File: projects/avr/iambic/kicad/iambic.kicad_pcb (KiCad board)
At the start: 2 copper layers, 48.3 x 50.8 mm, 24 parts, among them P1 CONN_1, P2 CONN_1, P3 CONN_1, P4 CONN_1, P5 CONN_1, P6 CONN_1, P7 CONN_1, P8 CONN_6, P9 CONN_1, Q1 NPN, Q2 NPN, U1 ATTINY45-20PU

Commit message: add install-op-rockpi/kicad/mp3server
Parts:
- RV1, RV2: footprint kicad:PIN_ARRAY_3X1 -> kicad:POT_V
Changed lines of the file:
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@@
     (add_net "Net-(R6-Pad1)")
   )
-  (module kicad:PIN_ARRAY_3X1 (layer F.Cu)
+  (module kicad:POT_V (layer F.Cu)
     (at 157.48 116.84 90)
     (descr "Connecteurs 2 pins")
@@
     )
   )
-  (module kicad:PIN_ARRAY_3X1 (layer F.Cu)
+  (module kicad:POT_V (layer F.Cu)
     (at 129.54 104.14 180)
     (descr "Connecteurs 2 pins")

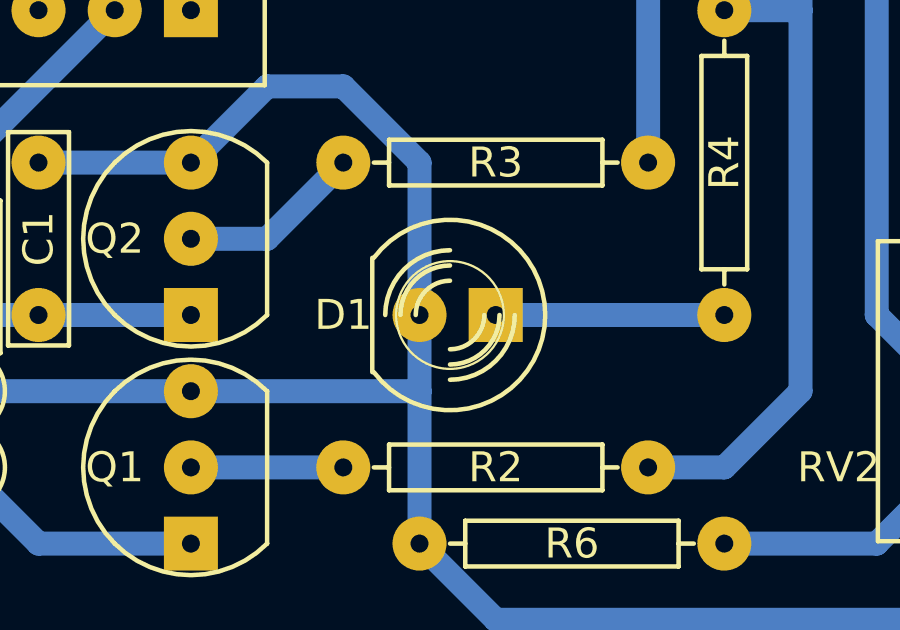
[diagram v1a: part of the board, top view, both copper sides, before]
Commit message: update kicad files
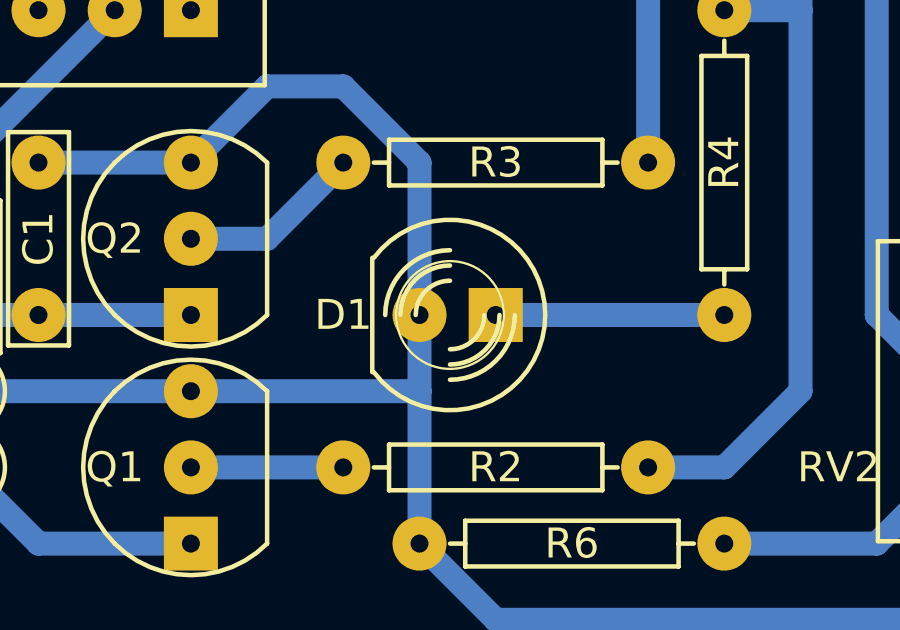
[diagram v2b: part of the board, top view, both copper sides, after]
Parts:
- C1, C2: footprint kicad:C2 -> common:C2
- D1: footprint kicad:LED-5MM -> common:LED-5MM
- LS1: footprint kicad:PIN_ARRAY_2X1 -> common:PIN_ARRAY_2X1
- P1, P2, P3, P4, P5, P6, P7, P9: footprint kicad:PIN_ARRAY_1X1 -> common:PIN_ARRAY_1X1
- P8: footprint kicad:PIN_ARRAY_6X1 -> common:PIN_ARRAY_6X1
- Q1, Q2: footprint kicad:NPN -> common:NPN
- R1, R2, R3, R4, R5, R6: footprint kicad:R4 -> common:R4
- RV1, RV2: footprint kicad:POT_V -> common:POT_V
- U1: footprint kicad:DIP-8__300 -> common:DIP-8__300
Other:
- net class Default removed
